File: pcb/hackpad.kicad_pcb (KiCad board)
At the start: 2 copper layers, 126.2 x 47.6 mm, 47 parts, among them SW1 SW_Push, SW10 SW_Push, SW11 RotaryEncoder_Switch, SW2 SW_Push, SW3 SW_Push, SW4 SW_Push, SW5 SW_Push, SW6 SW_Push, SW7 SW_Push, SW8 SW_Push, SW9 SW_Push, U1 XIAO-RP2040-DIP

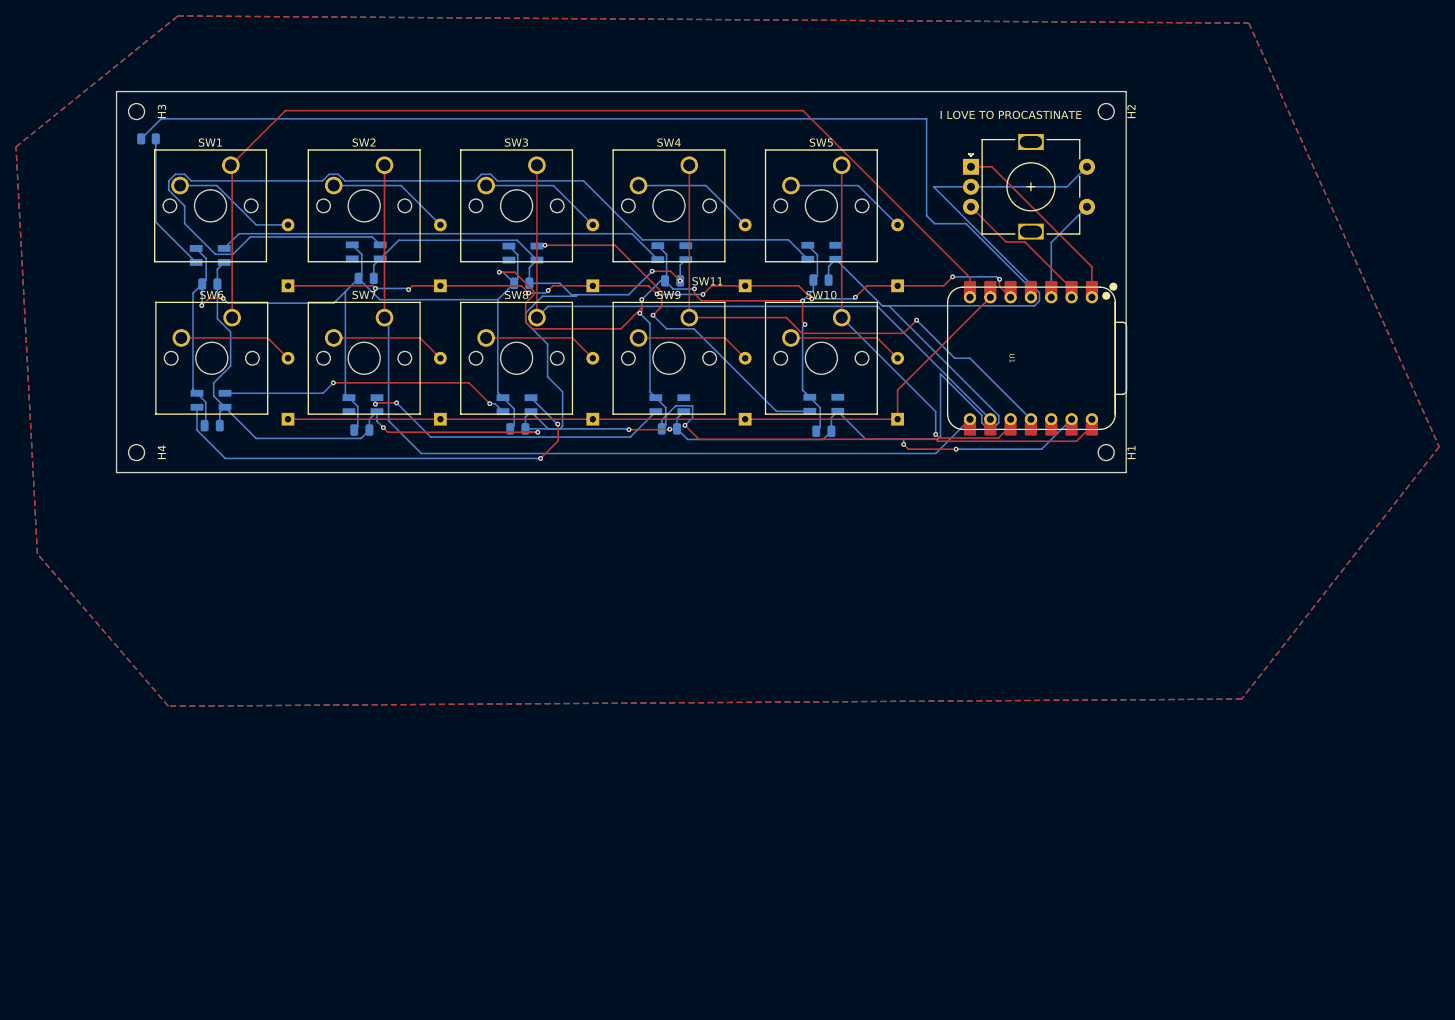
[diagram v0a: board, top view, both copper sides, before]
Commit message: Everything updated
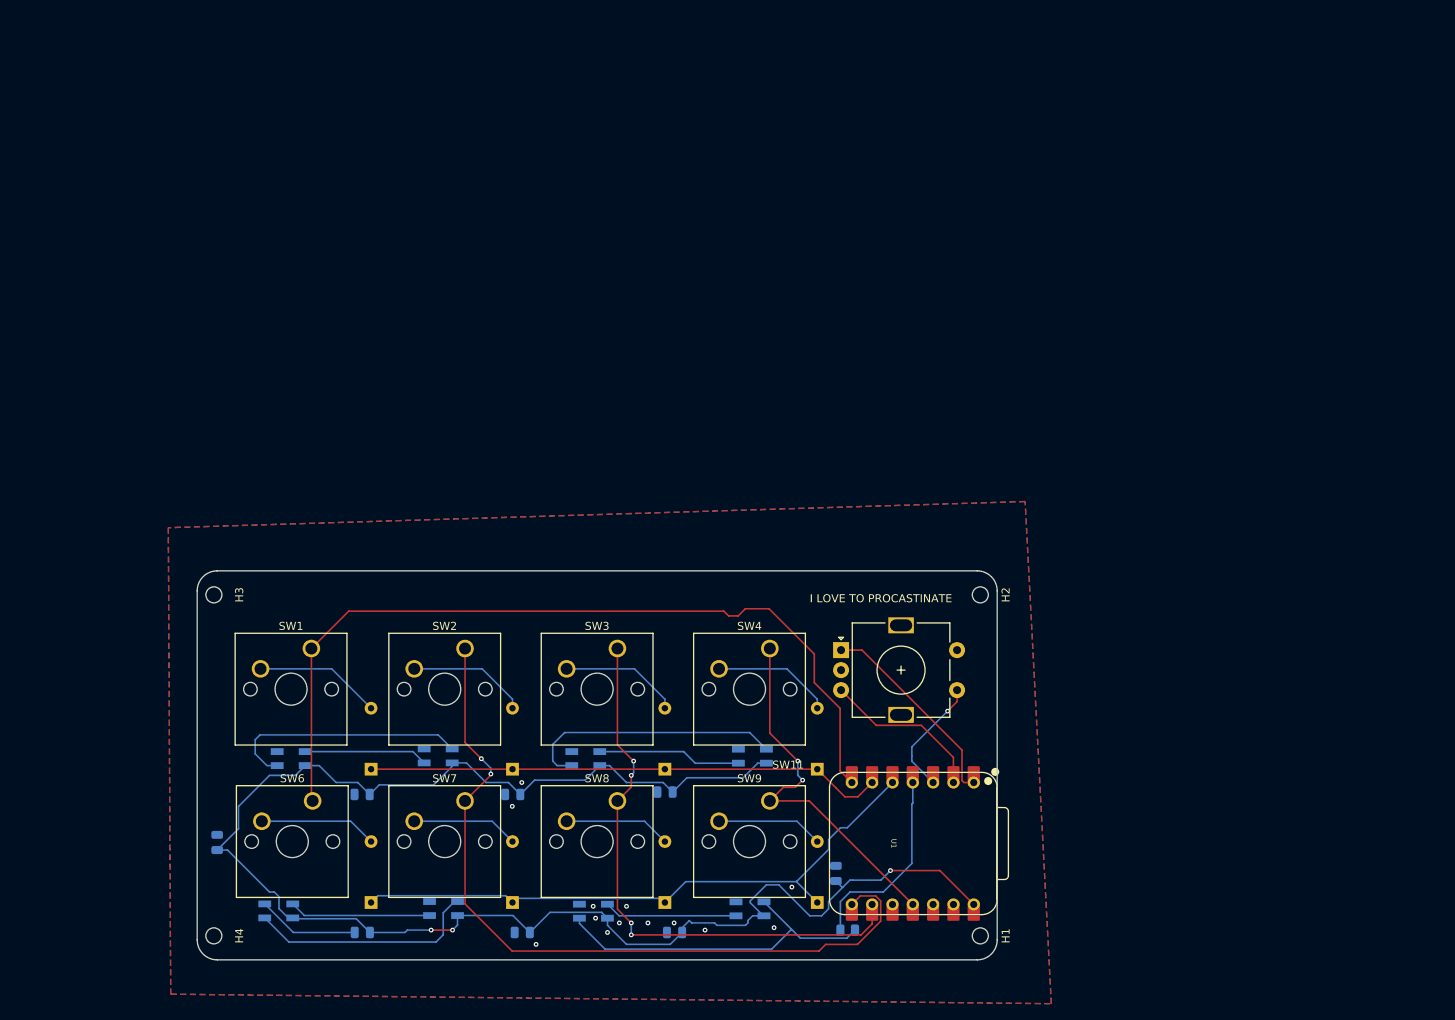
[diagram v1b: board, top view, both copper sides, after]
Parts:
- removed C10, C6: C, Capacitor_SMD:C_0805_2012Metric
- removed D10, D5: 1N4148, Diode_THT:D_DO-35_SOD27_P7.62mm_Horizontal
- removed D18, D20: SK6812MINI, LED_SMD:LED_SK6812MINI_PLCC4_3.5x3.5mm_P1.75mm
- removed SW10, SW5: SW_Push, Button_Switch_Keyboard:SW_Cherry_MX_1.00u_PCB
- moved R1 132.0 mm to (181.3, 144.9)
- moved D11 105.9 mm to (169.1, 142.2), turned to 0 degrees
- moved C1 99.7 mm to (159.7, 145.2), turned to 180 degrees
- moved C9 96.0 mm to (179.8, 137.8), turned to 90 degrees
- moved D16 93.0 mm to (110.2, 142.5), turned to 0 degrees
- moved C5 91.6 mm to (102.5, 134.0), turned to 90 degrees
- moved C2 84.0 mm to (140.6, 145.2), turned to 180 degrees
- moved C3 83.6 mm to (120.6, 145.2), turned to 180 degrees
- moved D14 82.9 mm to (149.5, 142.5), turned to 0 degrees
- moved D13 82.5 mm to (130.8, 142.2), turned to 0 degrees
- moved C4 75.0 mm to (120.6, 127.9), turned to 180 degrees
- moved D12 69.0 mm to (148.6, 123.5), turned to 0 degrees
- moved D15 63.6 mm to (169.4, 123.2), turned to 0 degrees
- moved SW11 62.6 mm to (188.0, 112.4)
- moved H2 62.4 mm to (197.9, 103.0)
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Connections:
- D12 pad 3: unconnected-(D12-DIN-Pad3) -> Net-(D12-DIN)
- D13 pad 3: unconnected-(D13-DIN-Pad3) -> Net-(D13-DIN)
- D14 pad 1: unconnected-(D14-DOUT-Pad1) -> Net-(D11-DIN)
- D15 pad 1: unconnected-(D15-DOUT-Pad1) -> Net-(D12-DIN)
- D16 pad 1: unconnected-(D16-DOUT-Pad1) -> Net-(D13-DIN)
- D17 pad 1: unconnected-(D17-DOUT-Pad1) -> Net-(D17-DOUT)
- D19 pad 3: unconnected-(D19-DIN-Pad3) -> Net-(D17-DOUT)
- U1 pad 10: Col 4 -> unconnected-(U1-GPIO4/MISO-Pad10)
- U1 pad 5: Row 0 -> Row 1
- U1 pad 6: Row 1 -> Row 0
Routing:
- net GND: track 345.4 -> 12.7 mm, vias 8 -> 13
- net LED: track 129.2 -> 24.6 mm
- net Net-(D12-DOUT): track 119.5 -> 32.9 mm
- net +5V: track 275.1 -> 205.2 mm, vias 9 -> 3
- net Net-(D18-DOUT): track 57.2 -> 0.00 mm, vias 2 -> 0
- net Col 4: track 48.7 -> 0.00 mm, vias 1 -> 0
- net Net-(D11-DOUT): track 56.3 -> 16.7 mm
- net Net-(D18-DIN): track 36.8 -> 0.00 mm, vias 2 -> 0
- net Row 0: track 95.7 -> 64.8 mm, vias 10 -> 0
- net Net-(D13-DIN): track 0.00 -> 29.1 mm
- net Net-(D13-DOUT): track 46.0 -> 17.7 mm, vias 2 -> 0
- net Net-(D11-DIN): track 17.5 -> 43.2 mm
- net Col 3: track 68.4 -> 46.6 mm, vias 1 -> 2
- net Col 0: track 125.4 -> 104.9 mm
- net Row 1: track 96.2 -> 76.9 mm
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- added copper zone on B.Cu, net GND
- added copper zone on F.Cu, net GND
- removed copper zone on B.Cu, net (none)
- removed copper zone on F.Cu, net (none)
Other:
- board size 126.2 x 47.6 mm -> 100 x 48.6 mm
